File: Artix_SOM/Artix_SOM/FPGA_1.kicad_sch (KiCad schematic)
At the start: 14 parts, among them SW1 SW_Push, U1 XC7A100T-FGG676

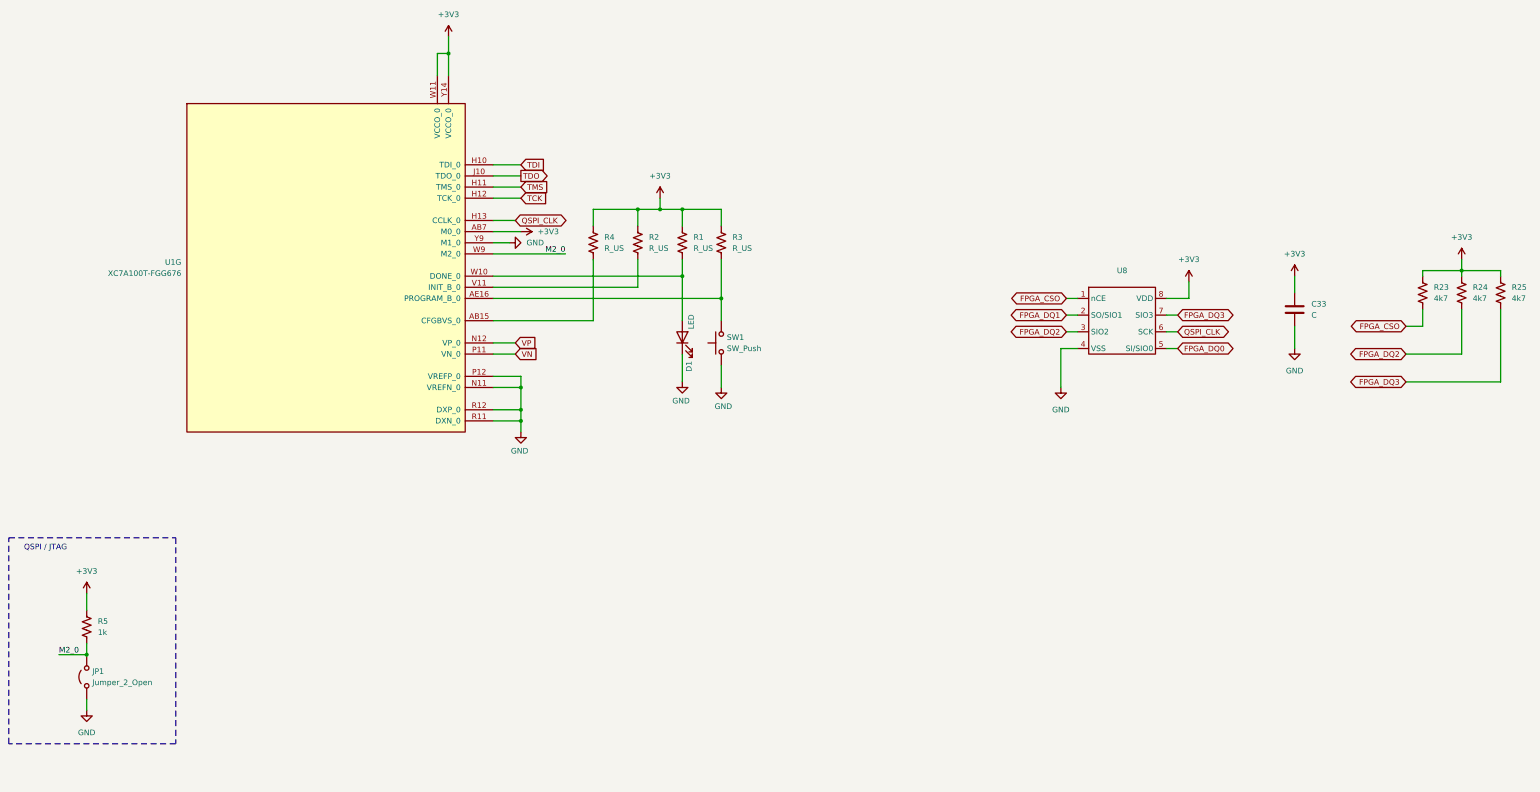
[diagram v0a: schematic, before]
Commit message: update
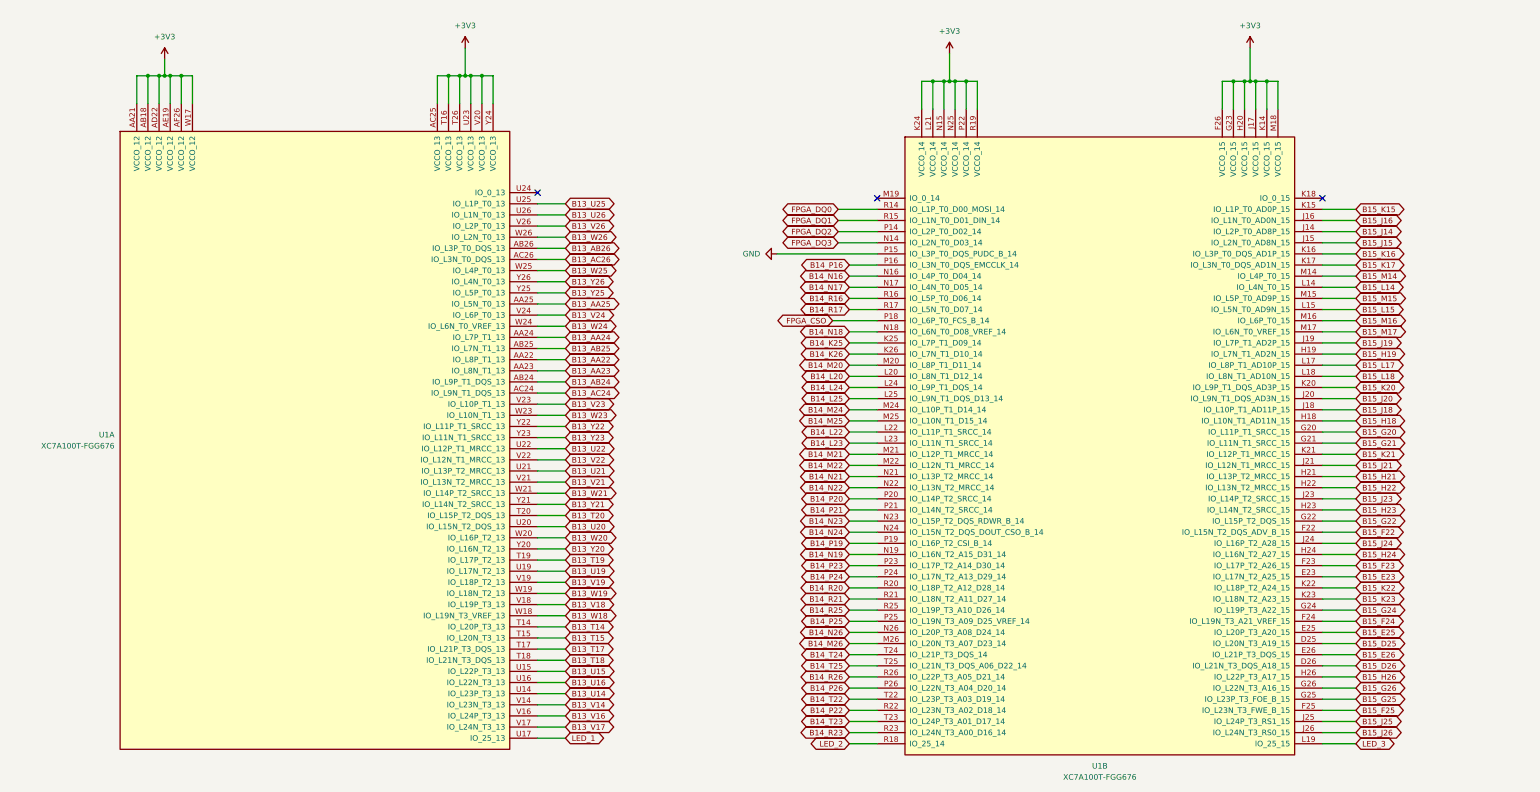
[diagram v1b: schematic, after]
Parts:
- removed C33: C, symbol Device:C
- removed D1: LED, symbol Device:LED
- removed JP1: Jumper_2_Open, symbol Jumper:Jumper_2_Open
- removed R1, R2, R3, R4: R_US, symbol Device:R_US
- removed R23, R24, R25: 4k7, symbol Device:R_US
- removed R5: 1k, symbol Device:R_US
- removed SW1: SW_Push, symbol Switch:SW_Push
- removed U1: XC7A100T-FGG676, symbol FPGA_Xilinx_Artix7:XC7A100T-FGG676
- removed U8: ~, symbol Sources:MT25QL128
- added U1: XC7A100T-FGG676, symbol FPGA_Xilinx_Artix7:XC7A100T-FGG676
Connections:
- net +3V3: now also U1.AA21 (VCCO_12), U1.AB18 (VCCO_12), U1.AC25 (VCCO_13), U1.AD22 (VCCO_12), U1.AE19 (VCCO_12), U1.AF26 (VCCO_12), U1.F26 (VCCO_15), U1.G23 (VCCO_15), U1.H20 (VCCO_15), U1.J17 (VCCO_15), U1.K14 (VCCO_15), U1.K24 (VCCO_14), U1.L21 (VCCO_14), U1.M18 (VCCO_15), U1.N15 (VCCO_14), U1.N25 (VCCO_14), U1.P22 (VCCO_14), U1.R19 (VCCO_14), U1.T16 (VCCO_13), U1.T26 (VCCO_13), U1.U23 (VCCO_13), U1.V20 (VCCO_13), U1.W17 (VCCO_12), U1.Y24 (VCCO_13)
- net FPGA_CSO: now also U1.P18 (IO_L6P_T0_FCS_B_14)
- net FPGA_DQ0: now also U1.R14 (IO_L1P_T0_D00_MOSI_14)
- net FPGA_DQ1: now also U1.R15 (IO_L1N_T0_D01_DIN_14)
- net FPGA_DQ2: now also U1.P14 (IO_L2P_T0_D02_14)
- net FPGA_DQ3: now also U1.N14 (IO_L2N_T0_D03_14)
- net GND: now also U1.P15 (IO_L3P_T0_DQS_PUDC_B_14)
- new net B13_AA22: U1.AA22 (IO_L8P_T1_13)
- new net B13_AA23: U1.AA23 (IO_L8N_T1_13)
- new net B13_AA24: U1.AA24 (IO_L7P_T1_13)
- new net B13_AA25: U1.AA25 (IO_L5N_T0_13)
- new net B13_AB24: U1.AB24 (IO_L9P_T1_DQS_13)
- new net B13_AB25: U1.AB25 (IO_L7N_T1_13)
- new net B13_AB26: U1.AB26 (IO_L3P_T0_DQS_13)
- new net B13_AC24: U1.AC24 (IO_L9N_T1_DQS_13)
- new net B13_AC26: U1.AC26 (IO_L3N_T0_DQS_13)
- new net B13_T14: U1.T14 (IO_L20P_T3_13)
- new net B13_T15: U1.T15 (IO_L20N_T3_13)
- new net B13_T17: U1.T17 (IO_L21P_T3_DQS_13)
- new net B13_T18: U1.T18 (IO_L21N_T3_DQS_13)
- new net B13_T19: U1.T19 (IO_L17P_T2_13)
- new net B13_T20: U1.T20 (IO_L15P_T2_DQS_13)
- new net B13_U14: U1.U14 (IO_L23P_T3_13)
- new net B13_U15: U1.U15 (IO_L22P_T3_13)
- new net B13_U16: U1.U16 (IO_L22N_T3_13)
- new net B13_U19: U1.U19 (IO_L17N_T2_13)
- new net B13_U20: U1.U20 (IO_L15N_T2_DQS_13)
- new net B13_U21: U1.U21 (IO_L13P_T2_MRCC_13)
- new net B13_U22: U1.U22 (IO_L12P_T1_MRCC_13)
- new net B13_U25: U1.U25 (IO_L1P_T0_13)
- new net B13_U26: U1.U26 (IO_L1N_T0_13)
- new net B13_V14: U1.V14 (IO_L23N_T3_13)
- new net B13_V16: U1.V16 (IO_L24P_T3_13)
- new net B13_V17: U1.V17 (IO_L24N_T3_13)
- new net B13_V18: U1.V18 (IO_L19P_T3_13)
- new net B13_V19: U1.V19 (IO_L18P_T2_13)
- new net B13_V21: U1.V21 (IO_L13N_T2_MRCC_13)
- new net B13_V22: U1.V22 (IO_L12N_T1_MRCC_13)
- new net B13_V23: U1.V23 (IO_L10P_T1_13)
- new net B13_V24: U1.V24 (IO_L6P_T0_13)
- new net B13_V26: U1.V26 (IO_L2P_T0_13)
- new net B13_W18: U1.W18 (IO_L19N_T3_VREF_13)
- new net B13_W19: U1.W19 (IO_L18N_T2_13)
- new net B13_W20: U1.W20 (IO_L16P_T2_13)
- new net B13_W21: U1.W21 (IO_L14P_T2_SRCC_13)
- new net B13_W23: U1.W23 (IO_L10N_T1_13)
- new net B13_W24: U1.W24 (IO_L6N_T0_VREF_13)
- new net B13_W25: U1.W25 (IO_L4P_T0_13)
- new net B13_W26: U1.W26 (IO_L2N_T0_13)
- new net B13_Y20: U1.Y20 (IO_L16N_T2_13)
- new net B13_Y21: U1.Y21 (IO_L14N_T2_SRCC_13)
- new net B13_Y22: U1.Y22 (IO_L11P_T1_SRCC_13)
- new net B13_Y23: U1.Y23 (IO_L11N_T1_SRCC_13)
- new net B13_Y25: U1.Y25 (IO_L5P_T0_13)
- new net B13_Y26: U1.Y26 (IO_L4N_T0_13)
- new net B14_K25: U1.K25 (IO_L7P_T1_D09_14)
- new net B14_K26: U1.K26 (IO_L7N_T1_D10_14)
- new net B14_L20: U1.L20 (IO_L8N_T1_D12_14)
- new net B14_L22: U1.L22 (IO_L11P_T1_SRCC_14)
- new net B14_L23: U1.L23 (IO_L11N_T1_SRCC_14)
- new net B14_L24: U1.L24 (IO_L9P_T1_DQS_14)
- new net B14_L25: U1.L25 (IO_L9N_T1_DQS_D13_14)
- new net B14_M20: U1.M20 (IO_L8P_T1_D11_14)
- new net B14_M21: U1.M21 (IO_L12P_T1_MRCC_14)
- new net B14_M22: U1.M22 (IO_L12N_T1_MRCC_14)
- new net B14_M24: U1.M24 (IO_L10P_T1_D14_14)
- new net B14_M25: U1.M25 (IO_L10N_T1_D15_14)
- new net B14_M26: U1.M26 (IO_L20N_T3_A07_D23_14)
- new net B14_N16: U1.N16 (IO_L4P_T0_D04_14)
- new net B14_N17: U1.N17 (IO_L4N_T0_D05_14)
- new net B14_N18: U1.N18 (IO_L6N_T0_D08_VREF_14)
- new net B14_N19: U1.N19 (IO_L16N_T2_A15_D31_14)
- new net B14_N21: U1.N21 (IO_L13P_T2_MRCC_14)
- new net B14_N22: U1.N22 (IO_L13N_T2_MRCC_14)
- new net B14_N23: U1.N23 (IO_L15P_T2_DQS_RDWR_B_14)
- new net B14_N24: U1.N24 (IO_L15N_T2_DQS_DOUT_CSO_B_14)
- new net B14_N26: U1.N26 (IO_L20P_T3_A08_D24_14)
- new net B14_P16: U1.P16 (IO_L3N_T0_DQS_EMCCLK_14)
- new net B14_P19: U1.P19 (IO_L16P_T2_CSI_B_14)
- new net B14_P20: U1.P20 (IO_L14P_T2_SRCC_14)
- new net B14_P21: U1.P21 (IO_L14N_T2_SRCC_14)
- new net B14_P22: U1.R22 (IO_L23N_T3_A02_D18_14)
- new net B14_P23: U1.P23 (IO_L17P_T2_A14_D30_14)
- new net B14_P24: U1.P24 (IO_L17N_T2_A13_D29_14)
- new net B14_P25: U1.P25 (IO_L19N_T3_A09_D25_VREF_14)
- new net B14_P26: U1.P26 (IO_L22N_T3_A04_D20_14)
- new net B14_R16: U1.R16 (IO_L5P_T0_D06_14)
- new net B14_R17: U1.R17 (IO_L5N_T0_D07_14)
- new net B14_R20: U1.R20 (IO_L18P_T2_A12_D28_14)
- new net B14_R21: U1.R21 (IO_L18N_T2_A11_D27_14)
- new net B14_R23: U1.R23 (IO_L24N_T3_A00_D16_14)
- new net B14_R25: U1.R25 (IO_L19P_T3_A10_D26_14)
- new net B14_R26: U1.R26 (IO_L22P_T3_A05_D21_14)
- new net B14_T22: U1.T22 (IO_L23P_T3_A03_D19_14)
- new net B14_T23: U1.T23 (IO_L24P_T3_A01_D17_14)
- new net B14_T24: U1.T24 (IO_L21P_T3_DQS_14)
- new net B14_T25: U1.T25 (IO_L21N_T3_DQS_A06_D22_14)
- new net B15_D25: U1.D25 (IO_L20N_T3_A19_15)
- new net B15_D26: U1.D26 (IO_L21N_T3_DQS_A18_15)
- new net B15_E23: U1.E23 (IO_L17N_T2_A25_15)
- new net B15_E25: U1.E25 (IO_L20P_T3_A20_15)
- new net B15_E26: U1.E26 (IO_L21P_T3_DQS_15)
- new net B15_F22: U1.F22 (IO_L15N_T2_DQS_ADV_B_15)
- new net B15_F23: U1.F23 (IO_L17P_T2_A26_15)
- new net B15_F24: U1.F24 (IO_L19N_T3_A21_VREF_15)
- new net B15_F25: U1.F25 (IO_L23N_T3_FWE_B_15)
- new net B15_G20: U1.G20 (IO_L11P_T1_SRCC_15)
- new net B15_G21: U1.G21 (IO_L11N_T1_SRCC_15)
- new net B15_G22: U1.G22 (IO_L15P_T2_DQS_15)
- new net B15_G24: U1.G24 (IO_L19P_T3_A22_15)
- new net B15_G25: U1.G25 (IO_L23P_T3_FOE_B_15)
- new net B15_G26: U1.G26 (IO_L22N_T3_A16_15)
- new net B15_H18: U1.H18 (IO_L10N_T1_AD11N_15)
- new net B15_H19: U1.H19 (IO_L7N_T1_AD2N_15)
- new net B15_H21: U1.H21 (IO_L13P_T2_MRCC_15)
- new net B15_H22: U1.H22 (IO_L13N_T2_MRCC_15)
- new net B15_H23: U1.H23 (IO_L14N_T2_SRCC_15)
- new net B15_H24: U1.H24 (IO_L16N_T2_A27_15)
- new net B15_H26: U1.H26 (IO_L22P_T3_A17_15)
- new net B15_J14: U1.J14 (IO_L2P_T0_AD8P_15)
- new net B15_J15: U1.J15 (IO_L2N_T0_AD8N_15)
- new net B15_J16: U1.J16 (IO_L1N_T0_AD0N_15)
- new net B15_J18: U1.J18 (IO_L10P_T1_AD11P_15)
- new net B15_J19: U1.J19 (IO_L7P_T1_AD2P_15)
- new net B15_J20: U1.J20 (IO_L9N_T1_DQS_AD3N_15)
- new net B15_J21: U1.J21 (IO_L12N_T1_MRCC_15)
- new net B15_J23: U1.J23 (IO_L14P_T2_SRCC_15)
- new net B15_J24: U1.J24 (IO_L16P_T2_A28_15)
- new net B15_J25: U1.J25 (IO_L24P_T3_RS1_15)
- new net B15_J26: U1.J26 (IO_L24N_T3_RS0_15)
- new net B15_K15: U1.K15 (IO_L1P_T0_AD0P_15)
- new net B15_K16: U1.K16 (IO_L3P_T0_DQS_AD1P_15)
- new net B15_K17: U1.K17 (IO_L3N_T0_DQS_AD1N_15)
- new net B15_K20: U1.K20 (IO_L9P_T1_DQS_AD3P_15)
- new net B15_K21: U1.K21 (IO_L12P_T1_MRCC_15)
- new net B15_K22: U1.K22 (IO_L18P_T2_A24_15)
- new net B15_K23: U1.K23 (IO_L18N_T2_A23_15)
- new net B15_L14: U1.L14 (IO_L4N_T0_15)
- new net B15_L15: U1.L15 (IO_L5N_T0_AD9N_15)
- new net B15_L17: U1.L17 (IO_L8P_T1_AD10P_15)
- new net B15_L18: U1.L18 (IO_L8N_T1_AD10N_15)
- new net B15_M14: U1.M14 (IO_L4P_T0_15)
- new net B15_M15: U1.M15 (IO_L5P_T0_AD9P_15)
- new net B15_M16: U1.M16 (IO_L6P_T0_15)
- new net B15_M17: U1.M17 (IO_L6N_T0_VREF_15)
- new net LED_1: U1.U17 (IO_25_13)
- new net LED_2: U1.R18 (IO_25_14)
- new net LED_3: U1.L19 (IO_25_15)
- no-connect marks 0 -> 3
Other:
- note removed: "QSPI / JTAG"
